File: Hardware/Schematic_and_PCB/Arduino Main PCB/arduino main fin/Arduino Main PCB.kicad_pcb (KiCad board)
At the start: 2 copper layers, 103.8 x 89.4 mm, 82 parts, among them J1 PIR_sensor, J10 LED_Room_2, J11 LED_Room_3, J12 LED_DOOR, J13 Buttons_Room_2, J14 Barrel_Jack, J15 Power switch, J2 Control_Panel, J3 Buttons_Room_3, J4 Buttons_Room_1, J5 Pot_Room_3.1, J6 Pot_Room_1, J7 Pot_Room_3.2, J8 LDR_Door, J9 LED_Room_1, Q1 BC557, Q2 BC557, Q3 BC557, Q4 BC557, Q5 BC557, Q6 BC557

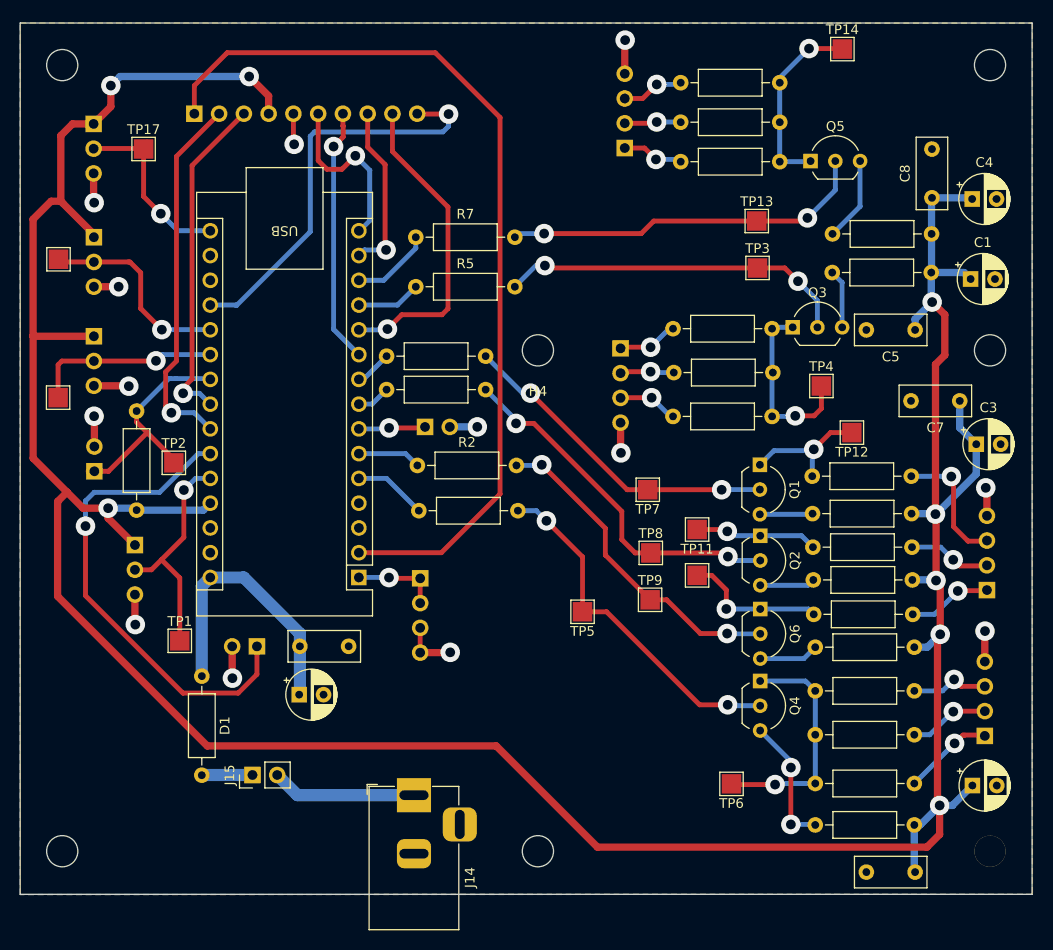
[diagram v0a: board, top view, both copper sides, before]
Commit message: Make schematic more readable.
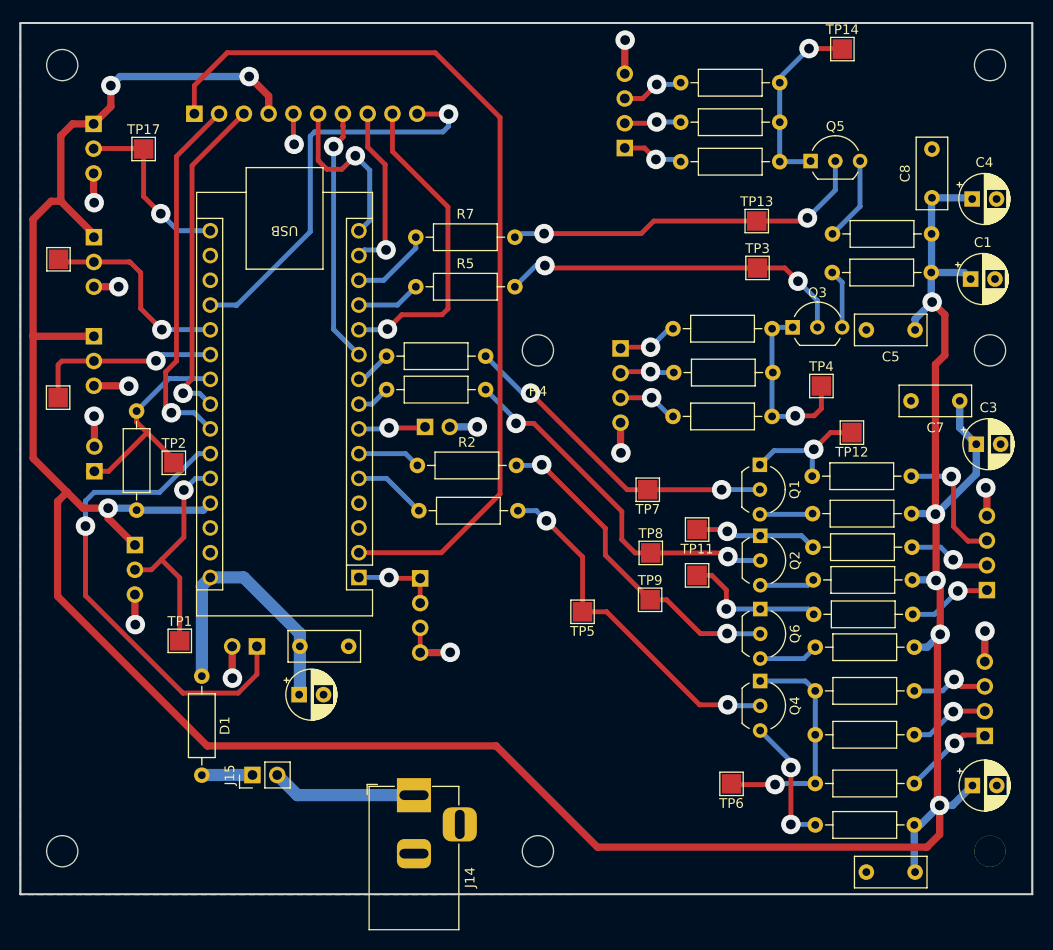
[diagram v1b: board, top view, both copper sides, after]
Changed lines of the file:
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@@
+	)
+	(gr_rect
+		(start 19.42 18.6625)
+		(end 123.21 108.0225)
+		(stroke
+			(width 0.2)
+			(type default)
+		)
+		(fill none)
+		(layer "Edge.Cuts")
 	)
 	(gr_rect
